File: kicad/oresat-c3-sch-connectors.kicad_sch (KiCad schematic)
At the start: 15 parts, among them J1 Conn_02x26_Odd_Even, J2 Conn_02x26_Odd_Even, J7 2-1734592-0

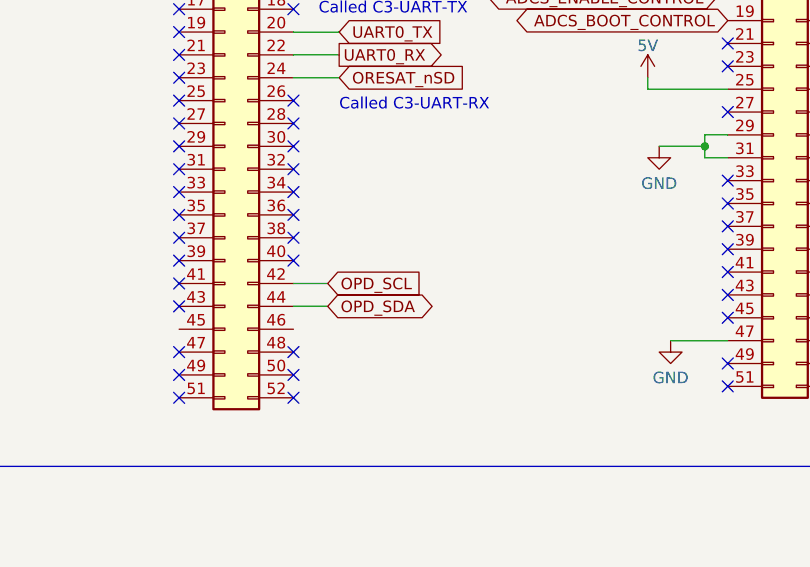
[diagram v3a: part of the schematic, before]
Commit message: Added UART TX pin for ADCS GNSS. Also fixed I2C SDA/SCL, they were swapped accidently
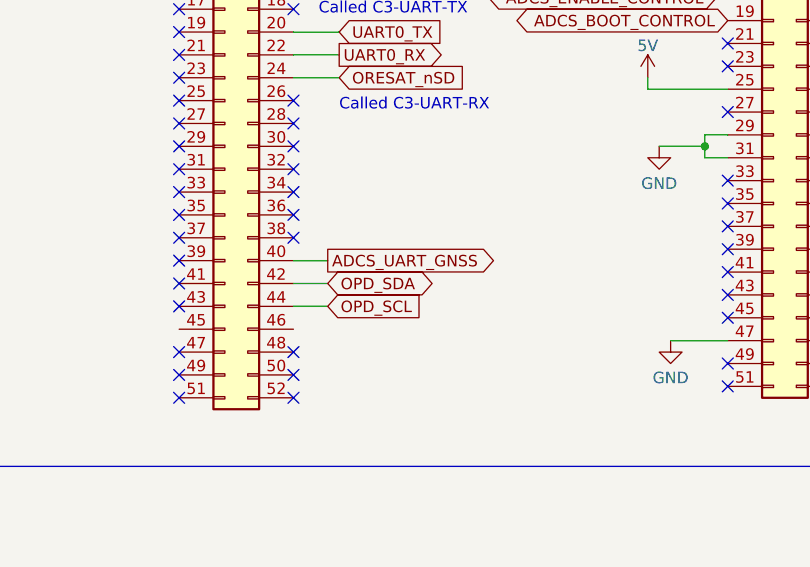
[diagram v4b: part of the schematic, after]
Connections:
- net OPD_SCL: now also J1.44 (Pin_44); no longer J1.42 (Pin_42)
- net OPD_SDA: now also J1.42 (Pin_42); no longer J1.44 (Pin_44)
- net ADCS_UART_GNSS: now reaches J1.40 (Pin_40)
- no-connect marks 90 -> 89
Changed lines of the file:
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@@
-	)
-	(no_connect
-		(at 125.73 105.41)
 	)
 	(no_connect
@@
 	(wire
 		(pts
+			(xy 274.32 130.81) (xy 262.89 130.81)
+		)
+		(stroke
+			(width 0)
+			(type default)
+		)
+	)
+	(wire
+		(pts
+			(xy 280.67 96.52) (xy 273.05 96.52)
+		)
+		(stroke
+			(width 0)
+			(type default)
+		)
+	)
+	(wire
+		(pts
+			(xy 279.4 73.66) (xy 280.67 73.66)
+		)
+		(stroke
+			(width 0)
+			(type default)
+		)
+	)
+	(wire
+		(pts
+			(xy 280.67 88.9) (xy 273.05 88.9)
+		)
+		(stroke
+			(width 0)
+			(type default)
+		)
+	)
+	(wire
+		(pts
+			(xy 125.73 110.49) (xy 129.54 110.49)
+		)
+		(stroke
+			(width 0)
+			(type default)
+		)
+	)
+	(wire
+		(pts
+			(xy 186.69 86.36) (xy 194.31 86.36)
+		)
+		(stroke
+			(width 0)
+			(type default)
+		)
+	)
+	(wire
+		(pts
+			(xy 171.45 91.44) (xy 171.45 92.71)
+		)
+		(stroke
+			(width 0)
+			(type default)
+		)
+	)
+	(wire
+		(pts
+			(xy 165.1 85.09) (xy 165.1 86.36)
+		)
+		(stroke
+			(width 0)
+			(type default)
+		)
+	)
+	(wire
+		(pts
+			(xy 186.69 71.12) (xy 191.77 71.12)
+		)
+		(stroke
+			(width 0)
+			(type default)
+		)
+	)
+	(wire
+		(pts
+			(xy 172.72 76.2) (xy 173.99 76.2)
+		)
+		(stroke
+			(width 0)
+			(type default)
+		)
+	)
+	(wire
+		(pts
+			(xy 130.81 80.01) (xy 125.73 80.01)
+		)
+		(stroke
+			(width 0)
+			(type default)
+		)
+	)
+	(wire
+		(pts
+			(xy 280.67 66.04) (xy 279.4 66.04)
+		)
+		(stroke
+			(width 0)
+			(type default)
+		)
+	)
+	(wire
+		(pts
+			(xy 273.05 114.3) (xy 275.59 114.3)
+		)
+		(stroke
+			(width 0)
+			(type default)
+		)
+	)
+	(wire
+		(pts
+			(xy 166.37 92.71) (xy 171.45 92.71)
+		)
+		(stroke
+			(width 0)
+			(type default)
+		)
+	)
+	(wire
+		(pts
+			(xy 125.73 105.41) (xy 129.54 105.41)
+		)
+		(stroke
+			(width 0)
+			(type default)
+		)
+	)
+	(wire
+		(pts
+			(xy 167.64 114.3) (xy 173.99 114.3)
+		)
+		(stroke
+			(width 0)
+			(type default)
+		)
+	)
+	(wire
+		(pts
+			(xy 173.99 91.44) (xy 171.45 91.44)
+		)
+		(stroke
+			(width 0)
+			(type default)
+		)
+	)
+	(wire
+		(pts
+			(xy 274.32 121.92) (xy 274.32 130.81)
+		)
+		(stroke
+			(width 0)
+			(type default)
+		)
+	)
+	(wire
+		(pts
+			(xy 280.67 93.98) (xy 273.05 93.98)
+		)
+		(stroke
+			(width 0)
+			(type default)
+		)
+	)
+	(wire
+		(pts
+			(xy 125.73 57.15) (xy 128.27 57.15)
+		)
+		(stroke
+			(width 0)
+			(type default)
+		)
+	)
+	(wire
+		(pts
 			(xy 125.73 107.95) (xy 129.54 107.95)
-		)
-		(stroke
-			(width 0)
-			(type default)
-		)
-	)
-	(wire
-		(pts
-			(xy 274.32 130.81) (xy 262.89 130.81)
-		)
-		(stroke
-			(width 0)
-			(type default)
-		)
-	)
-	(wire
-		(pts
-			(xy 280.67 96.52) (xy 273.05 96.52)
-		)
-		(stroke
-			(width 0)
-			(type default)
-		)
-	)
-	(wire
-		(pts
-			(xy 279.4 73.66) (xy 280.67 73.66)
-		)
-		(stroke
-			(width 0)
-			(type default)
-		)
-	)
-	(wire
-		(pts
-			(xy 280.67 88.9) (xy 273.05 88.9)
-		)
-		(stroke
-			(width 0)
-			(type default)
-		)
-	)
-	(wire
-		(pts
-			(xy 125.73 110.49) (xy 129.54 110.49)
-		)
-		(stroke
-			(width 0)
-			(type default)
-		)
-	)
-	(wire
-		(pts
-			(xy 186.69 86.36) (xy 194.31 86.36)
-		)
-		(stroke
-			(width 0)
-			(type default)
-		)
-	)
-	(wire
-		(pts
-			(xy 171.45 91.44) (xy 171.45 92.71)
-		)
-		(stroke
-			(width 0)
-			(type default)
-		)
-	)
-	(wire
-		(pts
-			(xy 165.1 85.09) (xy 165.1 86.36)
-		)
-		(stroke
-			(width 0)
-			(type default)
-		)
-	)
-	(wire
-		(pts
-			(xy 186.69 71.12) (xy 191.77 71.12)
-		)
-		(stroke
-			(width 0)
-			(type default)
-		)
-	)
-	(wire
-		(pts
-			(xy 172.72 76.2) (xy 173.99 76.2)
-		)
-		(stroke
-			(width 0)
-			(type default)
-		)
-	)
-	(wire
-		(pts
-			(xy 130.81 80.01) (xy 125.73 80.01)
-		)
-		(stroke
-			(width 0)
-			(type default)
-		)
-	)
-	(wire
-		(pts
-			(xy 280.67 66.04) (xy 279.4 66.04)
-		)
-		(stroke
-			(width 0)
-			(type default)
-		)
-	)
-	(wire
-		(pts
-			(xy 273.05 114.3) (xy 275.59 114.3)
-		)
-		(stroke
-			(width 0)
-			(type default)
-		)
-	)
-	(wire
-		(pts
-			(xy 166.37 92.71) (xy 171.45 92.71)
-		)
-		(stroke
-			(width 0)
-			(type default)
-		)
-	)
-	(wire
-		(pts
-			(xy 167.64 114.3) (xy 173.99 114.3)
-		)
-		(stroke
-			(width 0)
-			(type default)
-		)
-	)
-	(wire
-		(pts
-			(xy 173.99 91.44) (xy 171.45 91.44)
-		)
-		(stroke
-			(width 0)
-			(type default)
-		)
-	)
-	(wire
-		(pts
-			(xy 274.32 121.92) (xy 274.32 130.81)
-		)
-		(stroke
-			(width 0)
-			(type default)
-		)
-	)
-	(wire
-		(pts
-			(xy 280.67 93.98) (xy 273.05 93.98)
-		)
-		(stroke
-			(width 0)
-			(type default)
-		)
-	)
-	(wire
-		(pts
-			(xy 125.73 57.15) (xy 128.27 57.15)
 		)
 		(stroke
@@
 	(global_label "OPD_SDA"
 		(shape bidirectional)
-		(at 129.54 110.49 0)
-		(fields_autoplaced yes)
-		(effects
-			(font
-				(size 1.27 1.27)
-			)
-			(justify left)
-		)
-		(property "Intersheetrefs" "${INTERSHEET_REFS}"
-			(at 142.0427 110.49 0)
+		(at 129.54 107.95 0)
+		(fields_autoplaced yes)
+		(effects
+			(font
+				(size 1.27 1.27)
+			)
+			(justify left)
+		)
+		(property "Intersheetrefs" "${INTERSHEET_REFS}"
+			(at 142.0427 107.95 0)
 			(effects
 				(font
@@
 		)
 	)
+	(global_label "ADCS_UART_GNSS"
+		(shape output)
+		(at 129.54 105.41 0)
+		(fields_autoplaced yes)
+		(effects
+			(font
+				(size 1.27 1.27)
+			)
+			(justify left)
+		)
+		(property "Intersheetrefs" "${INTERSHEET_REFS}"
+			(at 148.9747 105.41 0)
+			(effects
+				(font
+					(size 1.27 1.27)
+				)
+				(justify left)
+			)
+		)
+	)
 	(global_label "UART0_RX"
 		(shape output)
@@
 	(global_label "OPD_SCL"
 		(shape input)
-		(at 129.54 107.95 0)
-		(fields_autoplaced yes)
-		(effects
-			(font
-				(size 1.27 1.27)
-			)
-			(justify left)
-		)
-		(property "Intersheetrefs" "${INTERSHEET_REFS}"
-			(at 140.8709 107.95 0)
-			(effects
-				(font
+		(at 129.54 110.49 0)
+		(fields_autoplaced yes)
+		(effects
+			(font
+				(size 1.27 1.27)
+			)
+			(justify left)
+		)
+		(property "Intersheetrefs" "${INTERSHEET_REFS}"
+			(at 140.8709 110.49 0)
+			(effects
+				(font

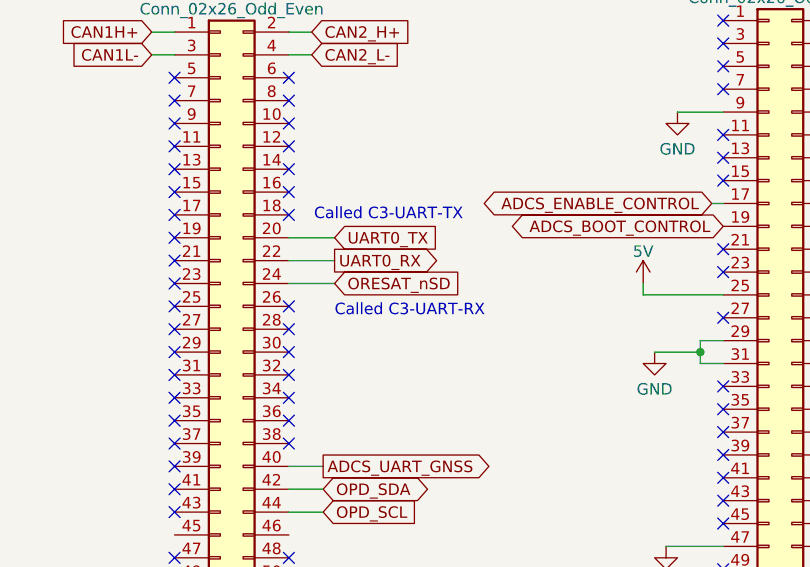
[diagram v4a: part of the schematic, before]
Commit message: Removed watchdog
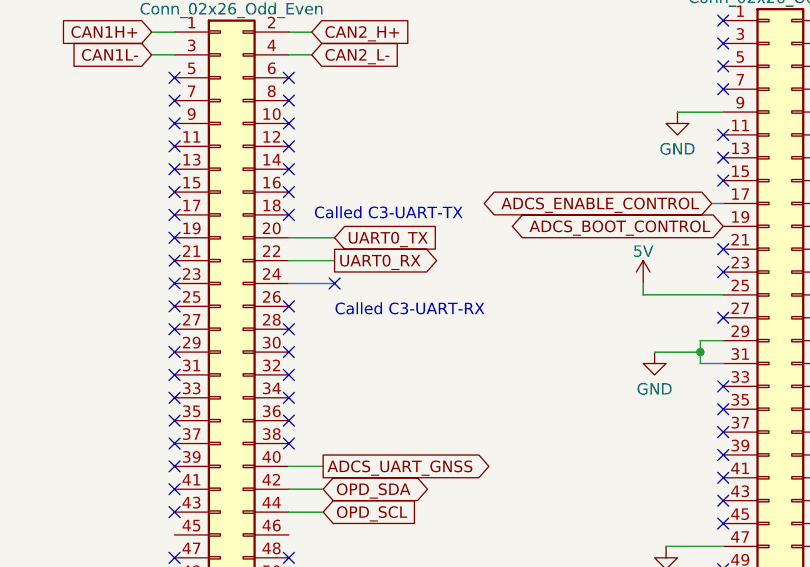
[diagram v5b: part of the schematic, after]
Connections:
- net ORESAT_nSD: no longer names the net of J1.24 (Pin_24)
- no-connect marks 89 -> 90
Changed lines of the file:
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@@
+	)
+	(no_connect
+		(at 130.81 85.09)
 	)
 	(no_connect
@@
 			(effects
 				(font
-					(size 1.27 1.27)
-				)
-				(justify left)
-			)
-		)
-	)
-	(global_label "ORESAT_nSD"
-		(shape input)
-		(at 130.81 85.09 0)
-		(fields_autoplaced yes)
-		(effects
-			(font
-				(size 1.27 1.27)
-			)
-			(justify left)
-		)
-		(property "Intersheetrefs" "${INTERSHEET_REFS}"
-			(at 145.3271 85.09 0)
-			(effects
-				(font

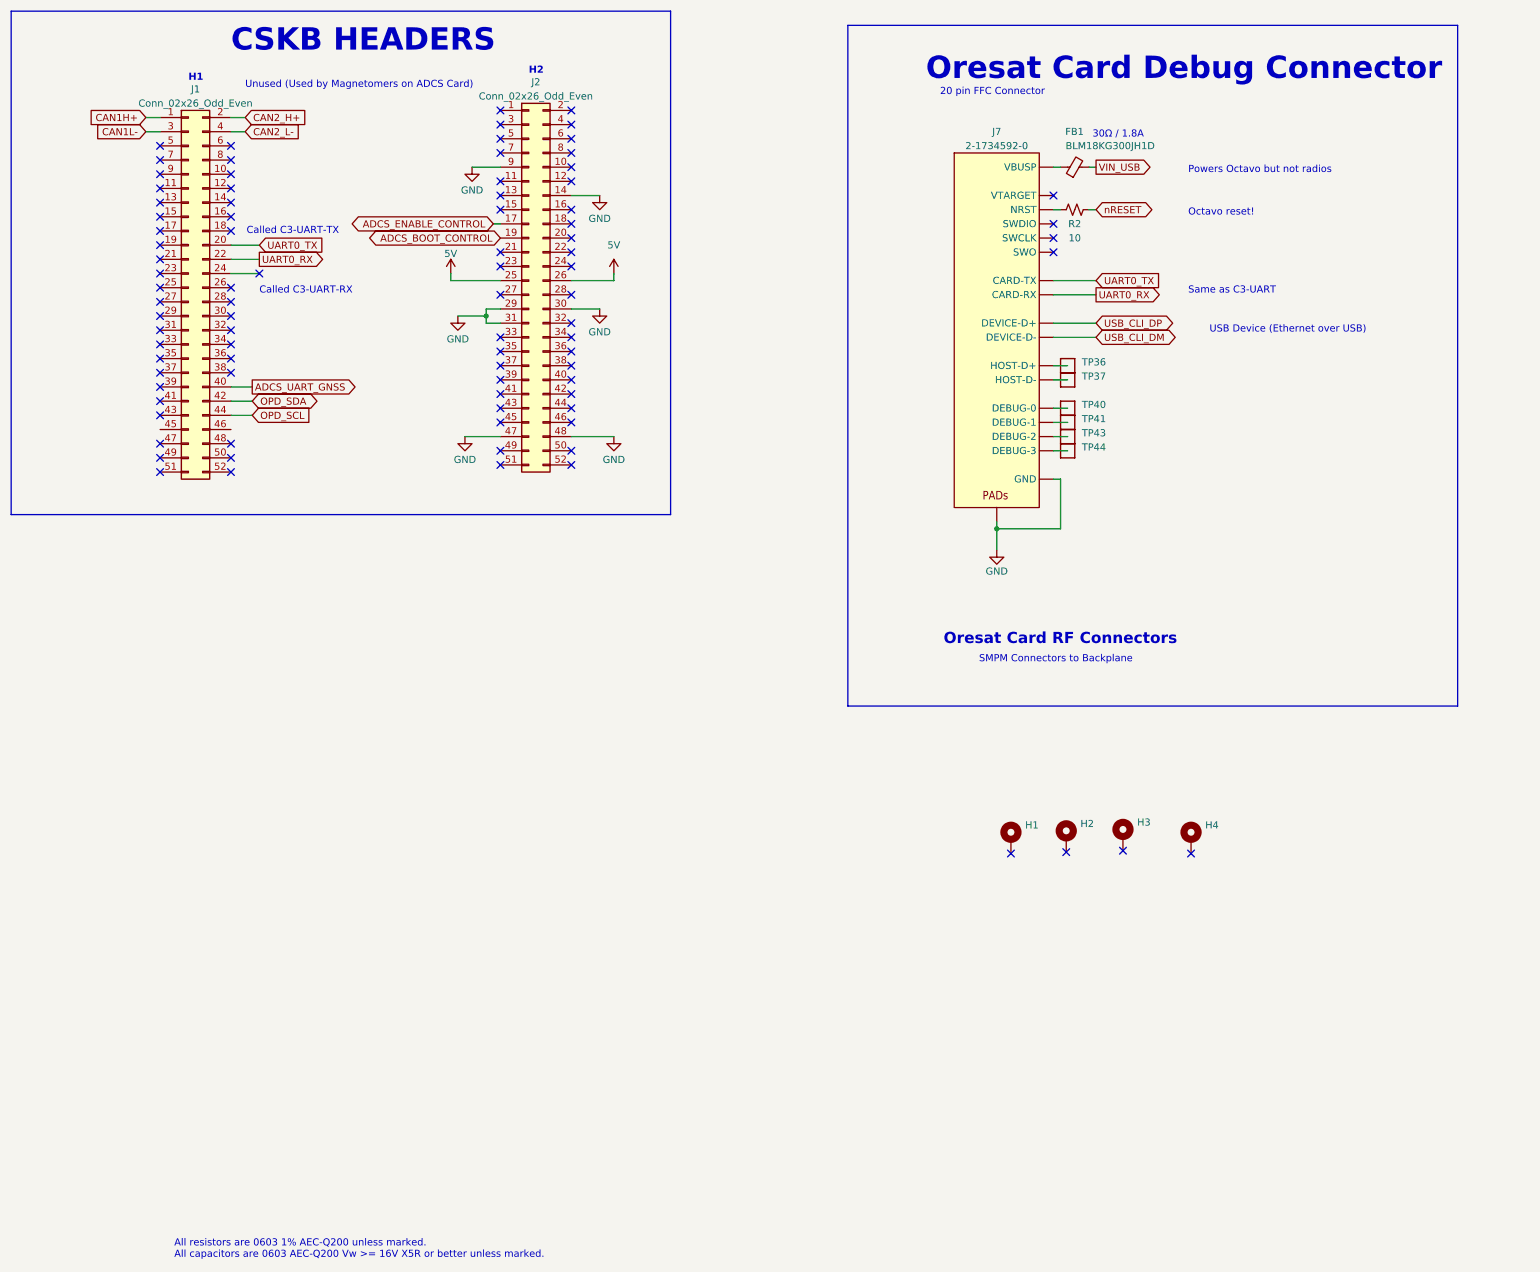
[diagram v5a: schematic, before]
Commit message: Added extra decoupling capacitor to MRAM. Also grounded all unused pins and mounting holes
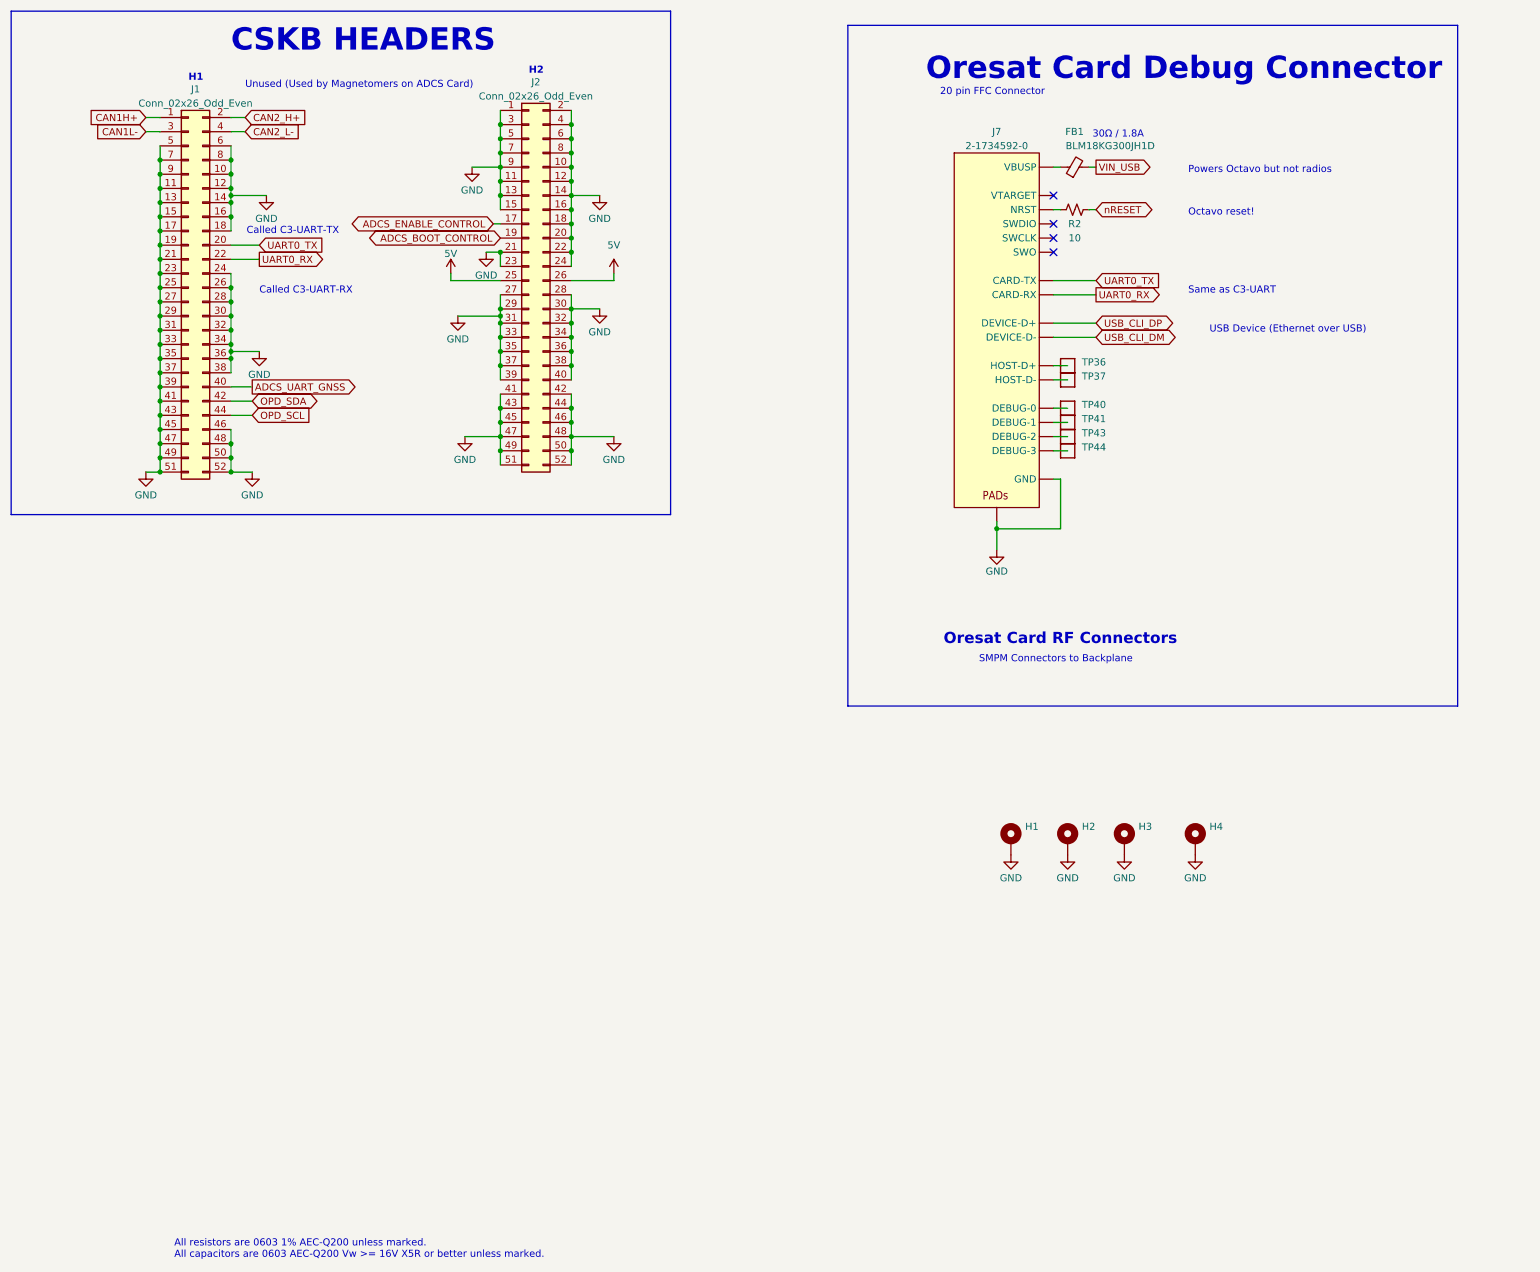
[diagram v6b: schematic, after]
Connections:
- net GND: now also H1.1, H2.1, H3.1, H4.1, J1.10 (Pin_10), J1.11 (Pin_11), J1.12 (Pin_12), J1.13 (Pin_13), J1.14 (Pin_14), J1.15 (Pin_15), J1.16 (Pin_16), J1.17 (Pin_17), J1.18 (Pin_18), J1.19 (Pin_19), J1.21 (Pin_21), J1.23 (Pin_23), J1.24 (Pin_24), J1.25 (Pin_25), J1.26 (Pin_26), J1.27 (Pin_27), J1.28 (Pin_28), J1.29 (Pin_29), J1.30 (Pin_30), J1.31 (Pin_31), J1.32 (Pin_32), J1.33 (Pin_33), J1.34 (Pin_34), J1.35 (Pin_35), J1.36 (Pin_36), J1.37 (Pin_37), J1.38 (Pin_38), J1.39 (Pin_39), J1.41 (Pin_41), J1.43 (Pin_43), J1.45 (Pin_45), J1.46 (Pin_46), J1.47 (Pin_47), J1.48 (Pin_48), J1.49 (Pin_49), J1.5 (Pin_5), J1.50 (Pin_50), J1.51 (Pin_51), J1.52 (Pin_52), J1.6 (Pin_6), J1.7 (Pin_7), J1.8 (Pin_8), J1.9 (Pin_9), J2.1 (Pin_1), J2.10 (Pin_10), J2.11 (Pin_11), J2.12 (Pin_12), J2.13 (Pin_13), J2.15 (Pin_15), J2.16 (Pin_16), J2.18 (Pin_18), J2.2 (Pin_2), J2.20 (Pin_20), J2.21 (Pin_21), J2.22 (Pin_22), J2.23 (Pin_23), J2.24 (Pin_24), J2.27 (Pin_27), J2.28 (Pin_28), J2.3 (Pin_3), J2.32 (Pin_32), J2.33 (Pin_33), J2.34 (Pin_34), J2.35 (Pin_35), J2.36 (Pin_36), J2.37 (Pin_37), J2.38 (Pin_38), J2.39 (Pin_39), J2.4 (Pin_4), J2.40 (Pin_40), J2.41 (Pin_41), J2.42 (Pin_42), J2.43 (Pin_43), J2.44 (Pin_44), J2.45 (Pin_45), J2.46 (Pin_46), J2.49 (Pin_49), J2.5 (Pin_5), J2.50 (Pin_50), J2.51 (Pin_51), J2.52 (Pin_52), J2.6 (Pin_6), J2.7 (Pin_7), J2.8 (Pin_8)
- no-connect marks 90 -> 4
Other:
- moved on the sheet: H2, H3, H4
